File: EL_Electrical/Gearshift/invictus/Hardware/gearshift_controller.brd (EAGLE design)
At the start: 66.4 x 62.4 mm, 69 parts, among them IC1 MCP2562-E_SN, IC2 MCP2515-I_SO, Q1 BSS138, Q10 BSS138, Q2 BSS138, Q3 BSS138, Q4 BSS138, Q5 BSS138, Q6 BSS138, Q8 BSS138, Q9 BSS138

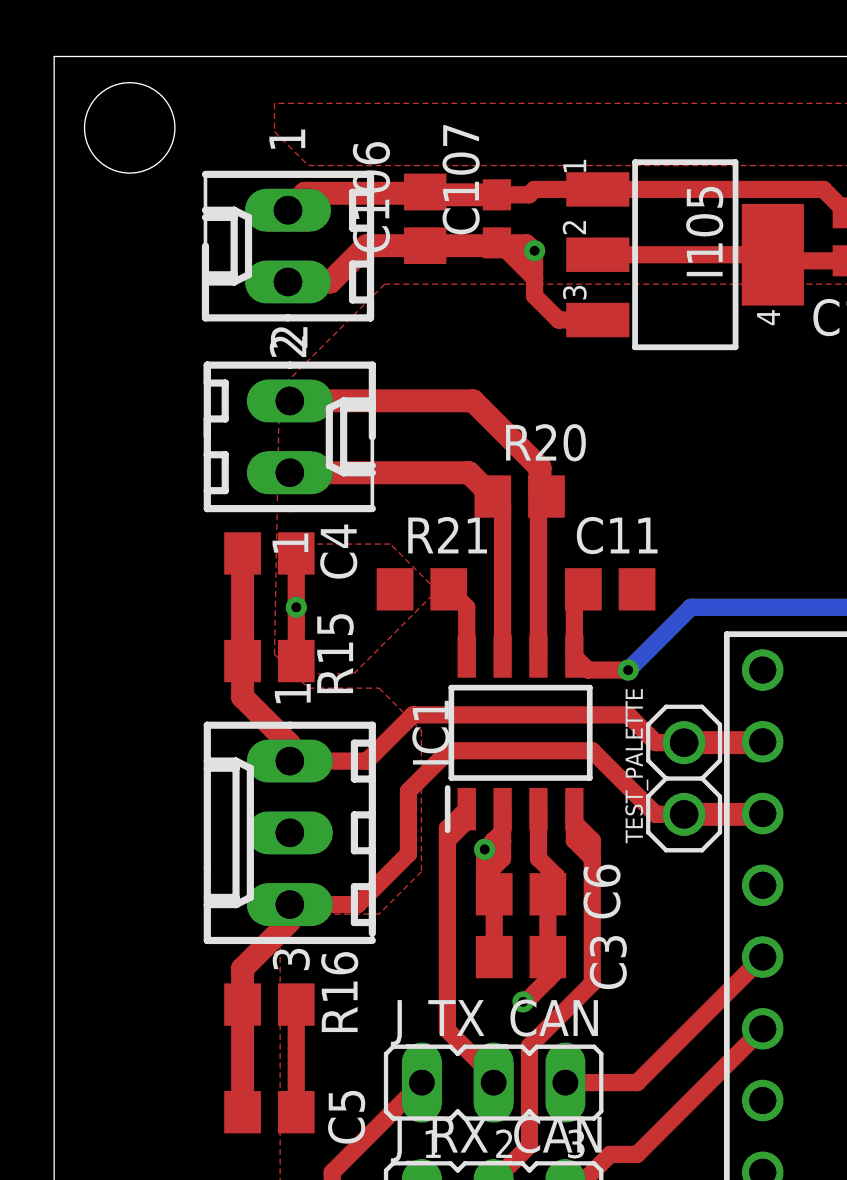
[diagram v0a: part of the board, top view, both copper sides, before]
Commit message: correction_final carte + fichier prod Cirly
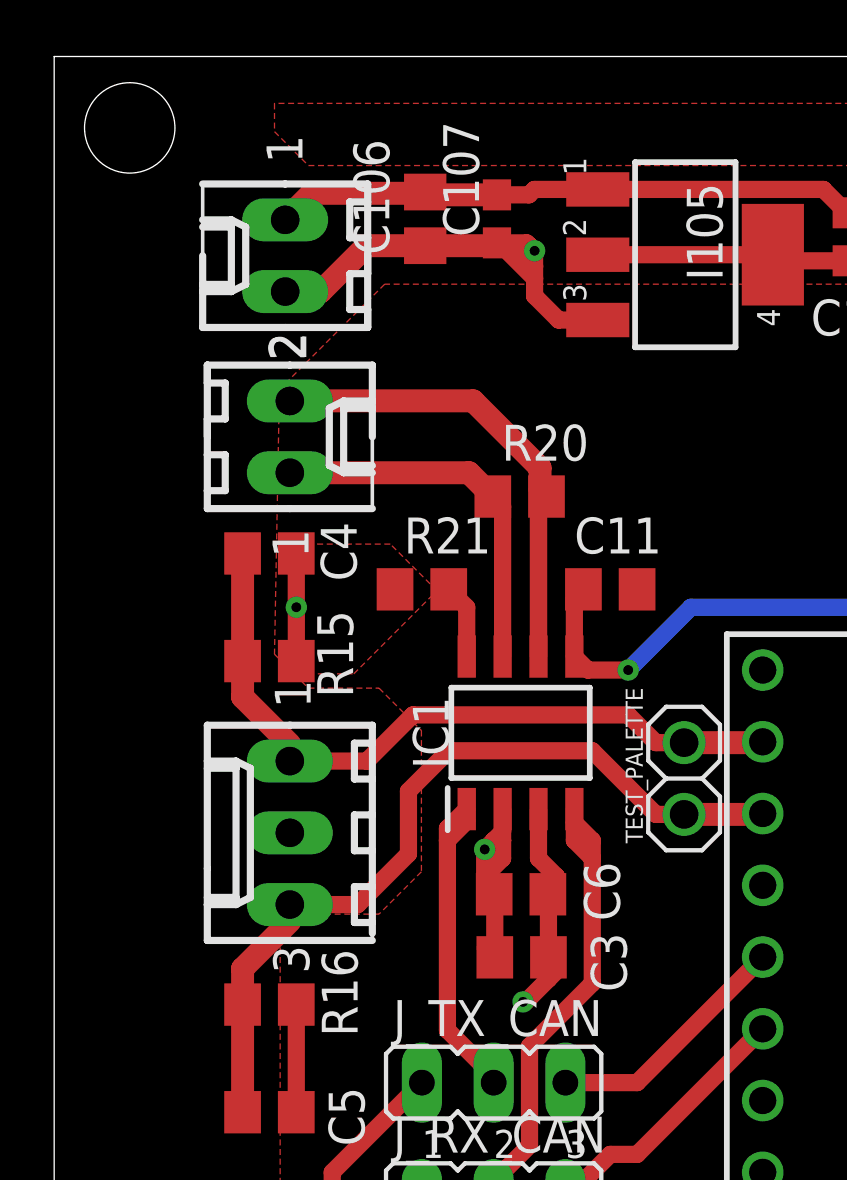
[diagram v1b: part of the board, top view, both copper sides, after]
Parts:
- moved POWER 0.35 mm to (8.18, 55.3)
